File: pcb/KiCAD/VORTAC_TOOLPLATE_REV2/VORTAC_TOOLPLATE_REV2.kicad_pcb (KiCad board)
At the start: 4 copper layers, 12.2 x 17 mm, 9 parts, among them J1 Conn_01x07, J2 Conn_01x02, J4 Conn_01x02, J5 Conn_01x03

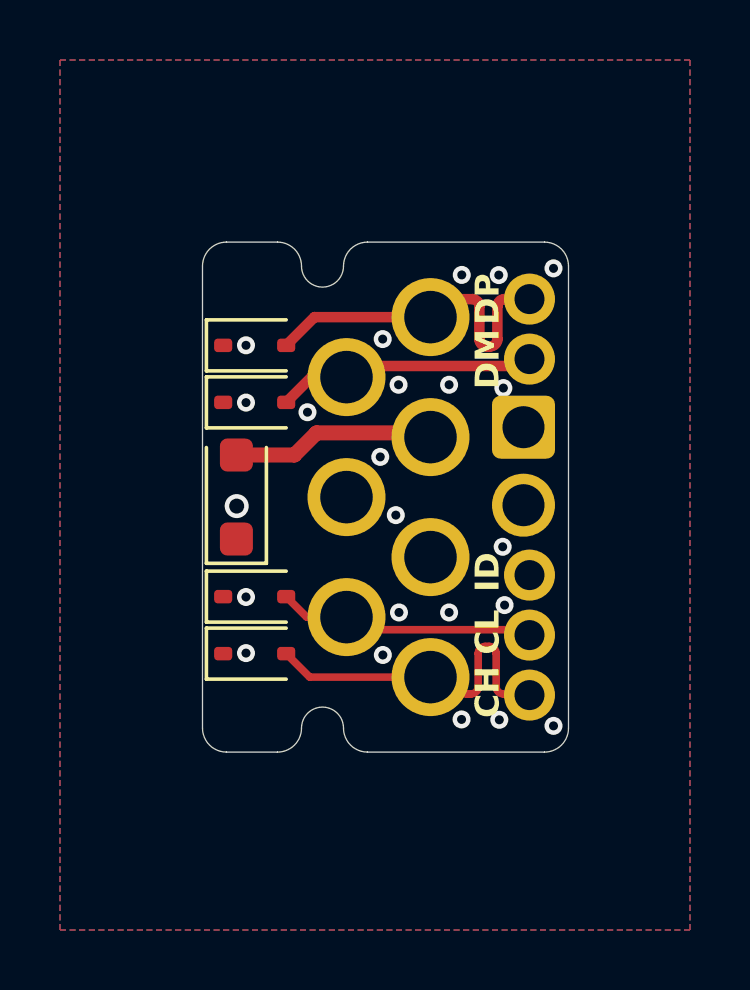
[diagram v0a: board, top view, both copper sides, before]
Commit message: Production Files
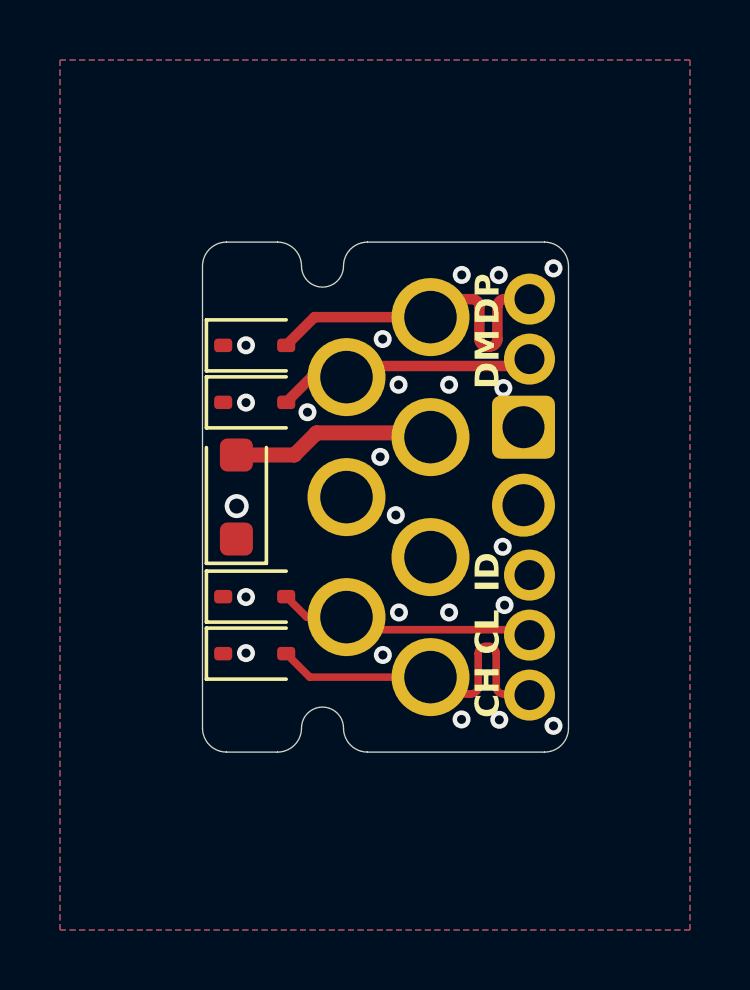
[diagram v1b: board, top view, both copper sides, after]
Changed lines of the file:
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@@
 	(gr_line
 		(start 107.8 91.499989)
-		(end 106.1 91.499989)
-		(stroke
-			(width 0.02)
-			(type default)
-		)
-		(layer "Edge.Cuts")
-	)
-	(gr_line
-		(start 110.8 91.5)
-		(end 110.8 91.499989)
+		(end 106.1 91.5)
 		(stroke
 			(width 0.02)
@@
 	(gr_line
 		(start 116.7 91.499989)
-		(end 110.8 91.499989)
+		(end 110.8 91.5)
 		(stroke
 			(width 0.02)
@@
 		(start 116.696001 108.499989)
 		(end 110.8 108.499989)
-		(stroke
-			(width 0.02)
-			(type default)
-		)
-		(layer "Edge.Cuts")
-	)
-	(gr_line
-		(start 106.1 91.5)
-		(end 106.1 91.499989)
 		(stroke
 			(width 0.02)
@@
 	)
 	(group ""
-		(members "189be37c-3439-4850-b8db-6974f42d414d" "1eb32afd-c09a-49d3-ae12-d6a83744d406"
-			"21ee54d1-b25d-440f-a083-593e3c46dabb" "242c97c3-1370-4787-8902-4c74beb9e0d2"
-			"288aa2d1-6382-4c43-be0d-32008cc0b90d" "350e9400-8a52-413e-ae4d-a73dbf6f3c46"
-			"4d014e9c-20f1-44d2-99bb-bf8e222ef4f6" "50010738-3090-489a-8392-c9fe1120f1c0"
-			"674f5e72-4eab-41f2-b3bd-86c1b8f001f9" "8648dc25-1319-4131-a77e-5e9f68fa7bdf"
-			"86fe878b-47ff-46c9-addd-8170ecce94a7" "b0bccc83-bd2c-4986-b417-d6d081e2046a"
-			"b4405535-8cd3-40de-9a75-9224b159281d" "c09d0ece-3274-46aa-b816-d19768a841f7"
-			"c848ccdf-6681-411e-ad1a-b1265674c511" "d23981ec-fc30-452c-ad1c-a582f1353f26"
-			"eb2d2922-3a95-453e-a3d7-e5c4d8309672" "ef064b4e-5029-4913-86ad-a9a4b9f7b6c1"
-		)
-	)
+		(members "189be37c-3439-4850-b8db-6974f42d414d" "21ee54d1-b25d-440f-a083-593e3c46dabb"
+			"242c97c3-1370-4787-8902-4c74beb9e0d2" "288aa2d1-6382-4c43-be0d-32008cc0b90d"
+			"350e9400-8a52-413e-ae4d-a73dbf6f3c46" "4d014e9c-20f1-44d2-99bb-bf8e222ef4f6"
+			"50010738-3090-489a-8392-c9fe1120f1c0" "674f5e72-4eab-41f2-b3bd-86c1b8f001f9"
+			"8648dc25-1319-4131-a77e-5e9f68fa7bdf" "86fe878b-47ff-46c9-addd-8170ecce94a7"
+			"b0bccc83-bd2c-4986-b417-d6d081e2046a" "b4405535-8cd3-40de-9a75-9224b159281d"
+			"c09d0ece-3274-46aa-b816-d19768a841f7" "c848ccdf-6681-411e-ad1a-b1265674c511"
+			"d23981ec-fc30-452c-ad1c-a582f1353f26" "eb2d2922-3a95-453e-a3d7-e5c4d8309672"
+		)
+	)
